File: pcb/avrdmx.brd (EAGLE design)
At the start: 53 x 60.9 mm, 15 parts, among them U1 ARDUINO_SHIELDLABEL

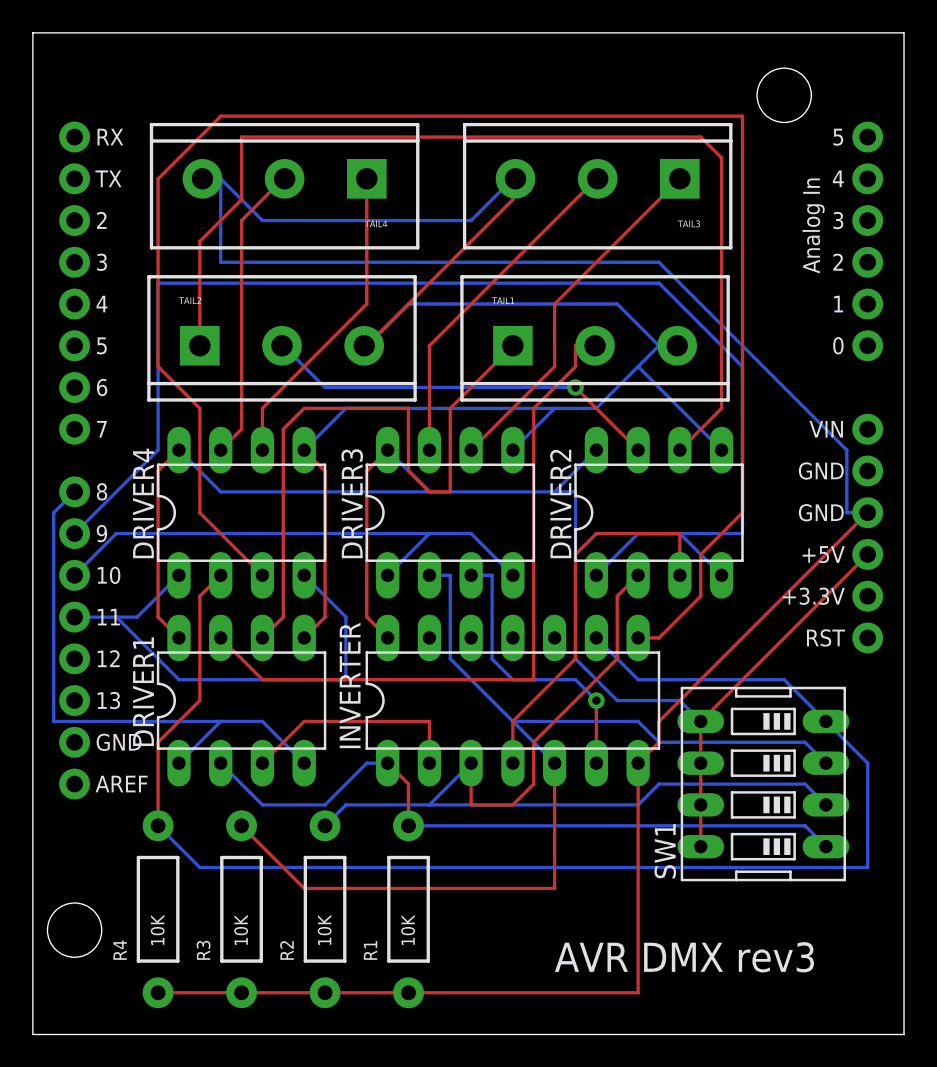
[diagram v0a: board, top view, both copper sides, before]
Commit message: schematic changes from a long time ago, not sure if they're good
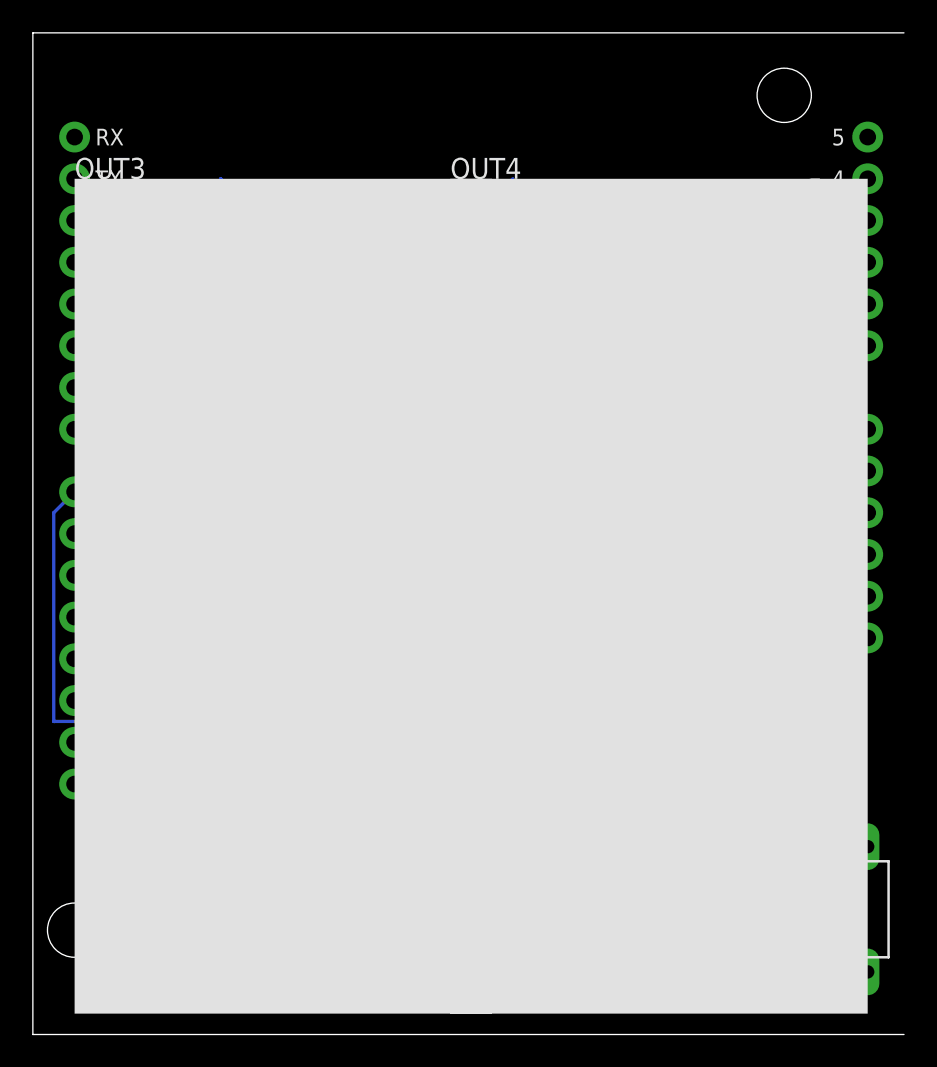
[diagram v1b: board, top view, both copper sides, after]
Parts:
- removed INVERTER: 7404N, 74xx-us:DIL14
- removed R1, R2, R3, R4: 10K, SparkFun-Resistors:AXIAL-0.4
- removed SW1: (no value), special:EDG-04
- removed TAIL1, TAIL2, TAIL3, TAIL4: (no value), SparkFun-Connectors:SCREWTERMINAL-5MM-3
- added DRIVER5: 75176AP, 751xx:DIL08
- added IR1: IR IN, pinhead:1X03
- added OUT1, OUT2, OUT3, OUT4: NC5FAV, avrdmx:NC5FAV
- added TAIL5: DMX IN, SparkFun-Connectors:SCREWTERMINAL-5MM-3
- moved DRIVER1 36.6 mm to (47.0, 27.9)
- moved DRIVER4 21.0 mm to (31.8, 43.2)
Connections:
- removed net N$17: DRIVER2.6, TAIL2.1
- removed net N$18: DRIVER2.7, TAIL2.2
- removed net N$19: DRIVER3.6, TAIL3.1
- removed net N$20: DRIVER3.7, TAIL3.2
- removed net N$21: DRIVER4.6, TAIL4.1
- removed net N$22: DRIVER4.7, TAIL4.2
- new net N$15: DRIVER4.6, OUT4.3
- new net N$6: DRIVER5.6, TAIL5.1
- net GND: now also DRIVER1.1, DRIVER2.1, DRIVER3.1, DRIVER4.1, DRIVER5.2, DRIVER5.3, DRIVER5.4, DRIVER5.5, IR1.2, OUT1.1, OUT2.1, OUT3.1, OUT4.1, TAIL5.3; no longer INVERTER.7, R1.P$1, R2.P$1, R3.P$1, R4.P$1, TAIL1.3, TAIL2.3, TAIL3.3, TAIL4.3
- net N$1: no longer DRIVER1.1
- net N$10: now also OUT1.3; no longer TAIL1.1
- net N$11: now also DRIVER2.7, OUT2.2; no longer DRIVER1.2, INVERTER.1, R1.P$2, SW1.1
- net N$12: now also DRIVER2.6, OUT2.3; no longer DRIVER2.2, INVERTER.3, R2.P$2, SW1.2
- net N$13: now also DRIVER3.7, OUT3.2; no longer DRIVER3.2, INVERTER.5, R3.P$2, SW1.3
- net N$14: now also DRIVER3.6, OUT3.3; no longer DRIVER4.2, INVERTER.9, R4.P$2, SW1.4
- net N$16: now also DRIVER4.7, OUT4.2; no longer DRIVER1.7, TAIL1.2
- net N$2: no longer DRIVER2.1
- net N$3: no longer DRIVER3.1
- net N$4: no longer DRIVER4.1
- net N$5: now also IR1.1, U1.D7; no longer DRIVER4.3, INVERTER.8
- net N$7: now also DRIVER5.7, TAIL5.2; no longer DRIVER3.3, INVERTER.6
- net N$8: now also DRIVER1.7, OUT1.2; no longer DRIVER2.3, INVERTER.4
- net N$9: now also DRIVER5.1, U1.RX; no longer DRIVER1.3, INVERTER.2
- net VCC: now also DRIVER1.2, DRIVER1.3, DRIVER2.2, DRIVER2.3, DRIVER3.2, DRIVER3.3, DRIVER4.2, DRIVER4.3, DRIVER5.8, IR1.3; no longer INVERTER.14, SW1.5, SW1.6, SW1.7, SW1.8
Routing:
- net GND: track 221.2 -> 107.9 mm
- net N$5: track 99.0 -> 0.00 mm
- net VCC: track 98.7 -> 0.00 mm
- net N$14: track 87.1 -> 0.00 mm
- net N$13: track 63.7 -> 0.00 mm
- net N$17: track 62.3 -> 0.00 mm
- net N$12: track 57.9 -> 0.00 mm
- net N$16: track 42.7 -> 0.00 mm
- net N$11: track 42.5 -> 0.00 mm
- net N$10: track 38.7 -> 0.00 mm
- net N$18: track 24.3 -> 0.00 mm, vias 1 -> 0
- net N$8: track 23.7 -> 0.00 mm
- net N$19: track 21.8 -> 0.00 mm
- net N$20: track 20.8 -> 0.00 mm
- net N$21: track 19.1 -> 0.00 mm
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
